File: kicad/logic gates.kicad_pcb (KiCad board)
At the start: 2 copper layers, 33 parts, among them J1 USB_B_Micro, Q1 NPN, Q2 NPN, Q3 NPN, Q4 NPN, Q5 NPN, Q6 NPN, Q7 NPN, SW1 SW_SPST, SW2 SW_SPST, SW3 SW_SPST, SW4 SW_SPST, SW5 SW_SPST, SW6 SW_SPST, SW7 SW_SPST, SW8 SW_DIP_x01

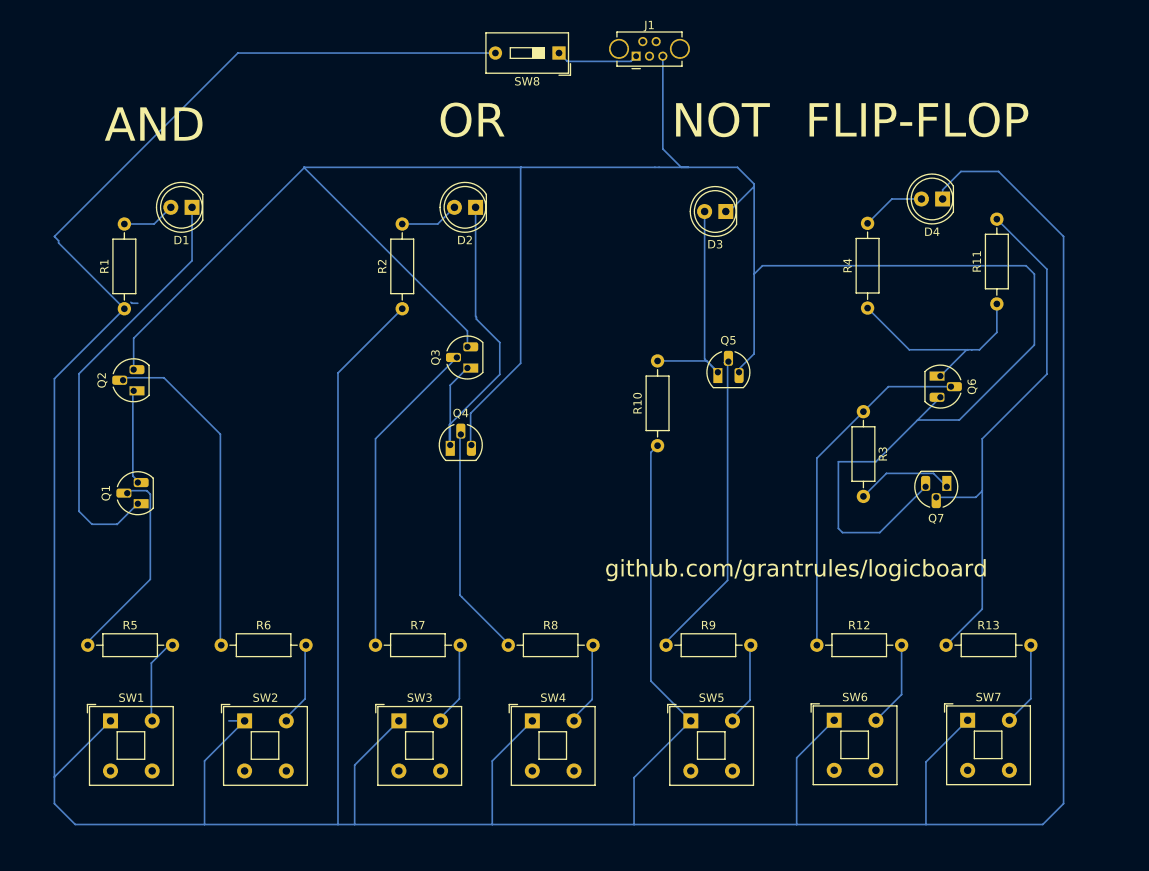
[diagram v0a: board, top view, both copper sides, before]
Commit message: fix pcb
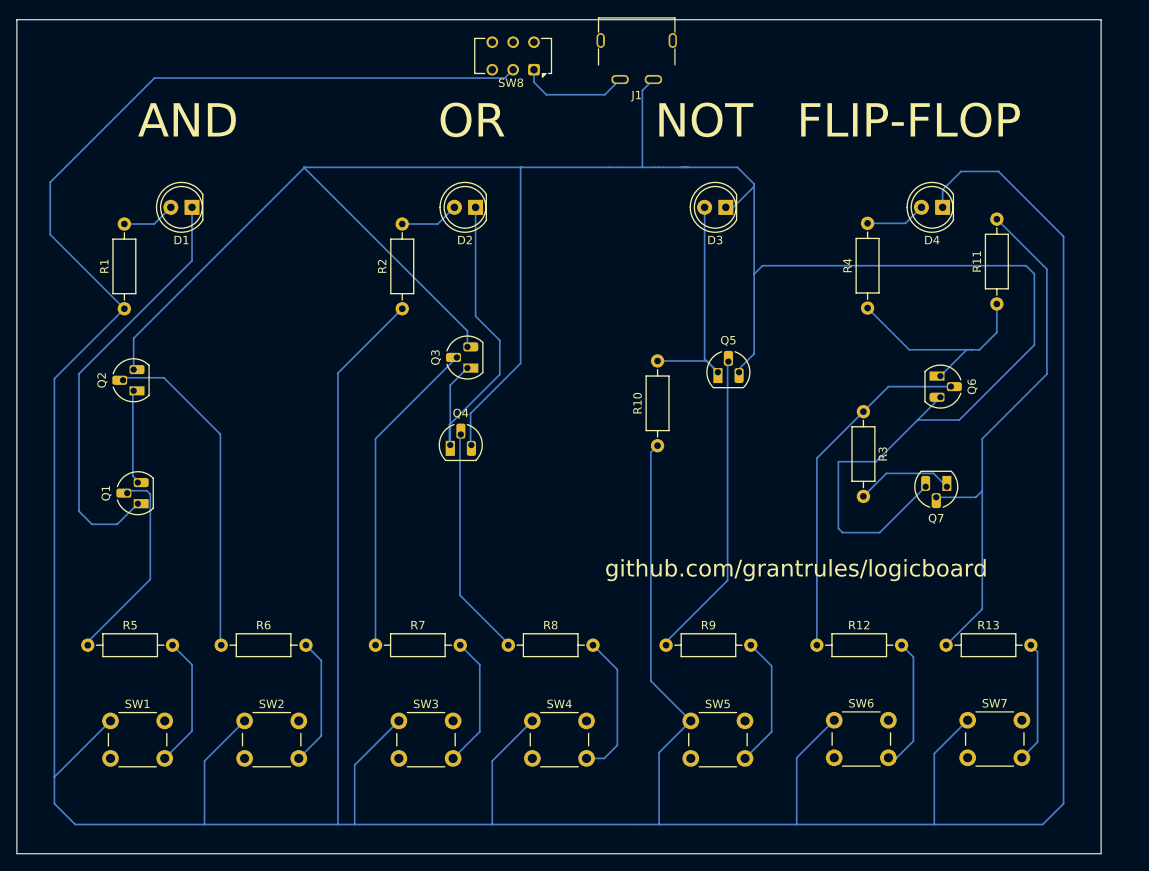
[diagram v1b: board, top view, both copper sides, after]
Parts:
- J1: value USB_B_Micro -> USB_C_2PIN; footprint Connector_USB:USB_Mini-B_Tensility_54-00023_Vertical_CircularHoles -> Aliexpress crap:USB_C_2pin-aliexpress
- SW1, SW2, SW3, SW4, SW5, SW6, SW7: footprint Button_Switch_THT:SW_Push_2P1T_Toggle_CK_PVA1xxH1xxxxxxV2 -> Button_Switch_THT:SW_PUSH_6mm_H5mm
- SW8: footprint Button_Switch_THT:SW_DIP_SPSTx01_Slide_9.78x4.72mm_W7.62mm_P2.54mm -> Button_Switch_THT:SW_CK_JS202011CQN_DPDT_Straight
- moved SW8 3.61 mm to (79.0, 18.0)
- moved D4 1.00 mm to (128.0, 34.5)
- moved J1 0.80 mm to (91.3, 15.6), turned to 180 degrees
- moved D3 0.50 mm to (102.0, 34.5)
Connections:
- SW8 pad 1: Net-(J1-VBUS) -> Net-(J1-GND)
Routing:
- net Net-(J1-GND): track 0.00 -> 13.2 mm
- net Net-(J1-VBUS): track 9.92 -> 0.00 mm
- net Net-(SW4-B): track 10.0 -> 17.6 mm
- net Net-(SW5-B): track 9.99 -> 15.9 mm
- net Net-(SW3-B): track 10.1 -> 15.9 mm
- net Net-(SW1-B): track 10.1 -> 15.9 mm
- net Net-(SW6-B): track 10.3 -> 15.9 mm
- net Net-(SW2-B): track 10.1 -> 15.5 mm
- net Net-(SW7-B): track 10.1 -> 14.6 mm
- net Net-(D4-K): track 547.7 -> 550.9 mm
- net Net-(D3-K): track 292.5 -> 289.4 mm
- net (no net): track 0.88 -> 0.00 mm
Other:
- board outline added: 130 x 100 mm
